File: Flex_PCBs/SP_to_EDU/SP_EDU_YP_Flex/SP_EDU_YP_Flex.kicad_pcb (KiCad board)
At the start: 2 copper layers, 4.5 x 64 mm, 2 parts, among them J1 Conn_01x08_Male, J2 Conn_01x08_Male

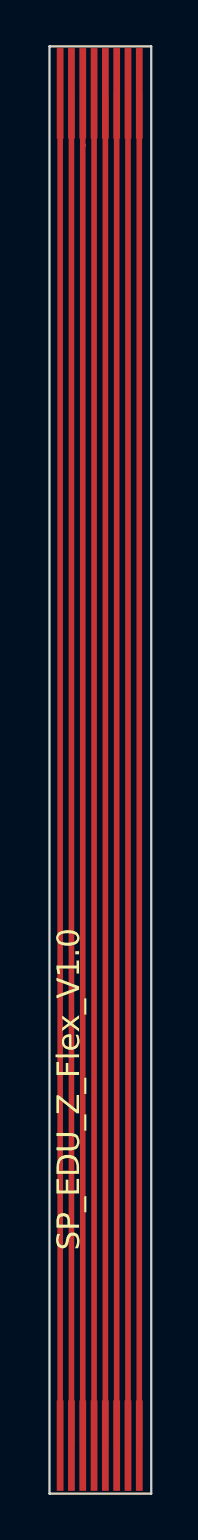
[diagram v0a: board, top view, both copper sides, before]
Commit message: Update SP_EDU_YP_Flex for FM
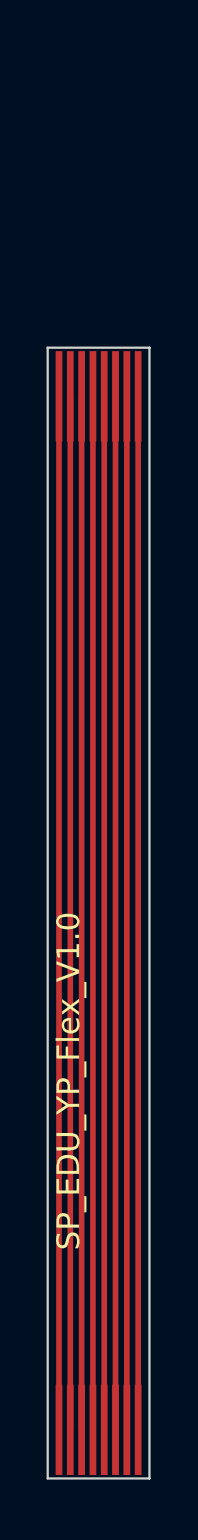
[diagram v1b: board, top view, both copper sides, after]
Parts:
- moved J1 13.4 mm to (123.0, 62.1)
- moved J2 0.70 mm to (127.5, 103.8)
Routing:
- net 8: track 59.8 -> 45.7 mm
- net 7: track 59.8 -> 45.7 mm
- net 5: track 59.8 -> 45.7 mm
- net 4: track 59.8 -> 45.7 mm
- net 3: track 59.8 -> 45.7 mm
- net 2: track 59.8 -> 45.7 mm
- net 1: track 59.8 -> 45.7 mm
- net 6: track 59.8 -> 45.7 mm
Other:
- board size 4.5 x 64 mm -> 4.5 x 50 mm
- board text added: "SP_EDU_YP_Flex_V1.0"
- board text removed: "SP_EDU_Z_Flex_V1.0"
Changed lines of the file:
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@@
 	(footprint "STS_connector:flexpcb con."
 		(layer "F.Cu")
-		(at 127.55 104.55 180)
+		(at 127.5 103.85 180)
 		(property "Reference" "J2"
 			(at -16.51 -3.81 180)
@@
 	(footprint "STS_connector:flexpcb con."
 		(layer "F.Cu")
-		(at 123.0508 48.75)
+		(at 123 62.15)
 		(property "Reference" "J1"
 			(at -16.51 -3.81 0)
@@
 	)
 	(gr_line
-		(start 123.079 108.6734)
-		(end 127.579 108.6734)
+		(start 123 108)
+		(end 127.5 108)
 		(stroke
 			(width 0.1)
@@
 	)
 	(gr_line
-		(start 123.079 44.6734)
-		(end 123.079 108.6734)
+		(start 123 58)
+		(end 123 108)
 		(stroke
 			(width 0.1)
@@
 	)
 	(gr_line
-		(start 123.079 44.6734)
-		(end 127.579 44.6734)
+		(start 123 58)
+		(end 127.5 58)
 		(stroke
 			(width 0.1)
@@
 	)
 	(gr_line
-		(start 127.579 44.6734)
-		(end 127.579 108.6734)
+		(start 127.5 58)
+		(end 127.5 108)
 		(stroke
 			(width 0.1)
@@
 	)
 	(gr_rect
-		(start 123.079 44.6734)
-		(end 127.579 52.1734)
+		(start 123 58)
+		(end 127.5 65.5)
 		(stroke
 			(width 0.15)
@@
 	)
 	(gr_rect
-		(start 123.1 101.2)
-		(end 127.6 108.7)
+		(start 123 100.5)
+		(end 127.5 108)
 		(stroke
 			(width 0.15)
@@
 		(layer "User.1")
 	)
-	(gr_text "SP_EDU_Z_Flex_V1.0"
+	(gr_text "SP_EDU_YP_Flex_V1.0"
 		(at 124.5108 97.917 90)
 		(layer "F.SilkS")
@@
 		(layer "User.1")
 		(pts
-			(xy 123.079 108.6734) (xy 123.079 44.7)
-		)
-		(height -6.329)
-		(gr_text "63,9734 mm"
-			(at 115.6 76.6867 90)
+			(xy 123 108) (xy 123 100.5)
+		)
+		(height -2.05)
+		(gr_text "7,5000 mm"
+			(at 119.8 104.25 90)
 			(layer "User.1")
 			(effects
@@
 			(extension_offset 0.5) keep_text_aligned)
 	)
-	(segment
-		(start 123.5508 106.5492)
-		(end 123.55 106.55)
+	(dimension
+		(type aligned)
+		(layer "User.1")
+		(pts
+			(xy 123.079 108) (xy 123.079 58)
+		)
+		(height -6.329)
+		(gr_text "50,0000 mm"
+			(at 115.6 83 90)
+			(layer "User.1")
+			(effects
+				(font
+					(size 1 1)
+					(thickness 0.15)
+				)
+			)
+		)
+		(format
+			(prefix "")
+			(suffix "")
+			(units 3)
+			(units_format 1)
+			(precision 4)
+		)
+		(style
+			(thickness 0.15)
+			(arrow_length 1.27)
+			(text_position_mode 0)
+			(extension_height 0.58642)
+			(extension_offset 0.5) keep_text_aligned)
+	)
+	(segment
+		(start 123.5 60.15)
+		(end 123.5 105.85)
 		(width 0.25)
 		(layer "F.Cu")
@@
 	)
 	(segment
-		(start 123.5508 46.75)
-		(end 123.5508 106.5492)
-		(width 0.25)
-		(layer "F.Cu")
-		(net 1)
-	)
-	(segment
-		(start 124.05 106.55)
-		(end 124.05 46.7508)
+		(start 124 105.85)
+		(end 124 60.15)
 		(width 0.25)
 		(layer "F.Cu")
@@
 	)
 	(segment
-		(start 124.05 46.7508)
-		(end 124.0508 46.75)
-		(width 0.25)
-		(layer "F.Cu")
-		(net 2)
-	)
-	(segment
-		(start 124.55 49.0508)
-		(end 124.55 106.55)
+		(start 124.5 60.15)
+		(end 124.5 105.85)
 		(width 0.25)
 		(layer "F.Cu")
@@
 	)
 	(segment
-		(start 124.5508 49.05)
-		(end 124.55 49.0508)
-		(width 0.25)
-		(layer "F.Cu")
-		(net 3)
-	)
-	(segment
-		(start 124.5508 46.75)
-		(end 124.5508 49.05)
-		(width 0.25)
-		(layer "F.Cu")
-		(net 3)
-	)
-	(segment
-		(start 125.05 106.55)
-		(end 125.05 46.7508)
+		(start 125 105.85)
+		(end 125 60.15)
 		(width 0.25)
 		(layer "F.Cu")
@@
 	)
 	(segment
-		(start 125.05 46.7508)
-		(end 125.0508 46.75)
-		(width 0.25)
-		(layer "F.Cu")
-		(net 4)
-	)
-	(segment
-		(start 125.5508 46.75)
-		(end 125.5508 106.5492)
+		(start 125.5 60.15)
+		(end 125.5 105.85)
 		(width 0.25)
 		(layer "F.Cu")
@@
 	)
 	(segment
-		(start 125.5508 106.5492)
-		(end 125.55 106.55)
-		(width 0.25)
-		(layer "F.Cu")
-		(net 5)
-	)
-	(segment
-		(start 126.05 106.55)
-		(end 126.05 46.7508)
+		(start 126 105.85)
+		(end 126 60.15)
 		(width 0.25)
 		(layer "F.Cu")
@@
 	)
 	(segment
-		(start 126.05 46.7508)
-		(end 126.0508 46.75)
-		(width 0.25)
-		(layer "F.Cu")
-		(net 6)
-	)
-	(segment
-		(start 126.5508 46.75)
-		(end 126.5508 106.5492)
+		(start 126.5 60.15)
+		(end 126.5 105.85)
 		(width 0.25)
 		(layer "F.Cu")
@@
 	)
 	(segment
-		(start 126.5508 106.5492)
-		(end 126.55 106.55)
-		(width 0.25)
-		(layer "F.Cu")
-		(net 7)
-	)
-	(segment
-		(start 127.05 106.55)
-		(end 127.05 46.7508)
-		(width 0.25)
-		(layer "F.Cu")
-		(net 8)
-	)
-	(segment
-		(start 127.05 46.7508)
-		(end 127.0508 46.75)
-		(width 0.25)
-		(layer "F.Cu")
+		(start 127 105.85)
+		(end 127 60.15)
+		(width 0.25)
+		(layer "F.Cu")
